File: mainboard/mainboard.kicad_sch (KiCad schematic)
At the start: 46 parts, among them J1 Conn_01x14, J2 Conn_02x06_Top_Bottom, J3 OLED, J6 Conn_01x05, J7 SHF-105-01-L-D-RA, SW35 SW_Push, SW36 SW_Push, U1 RP2350A, U2 W25Q128JVSIQ, Y1 ABM8-272-T3

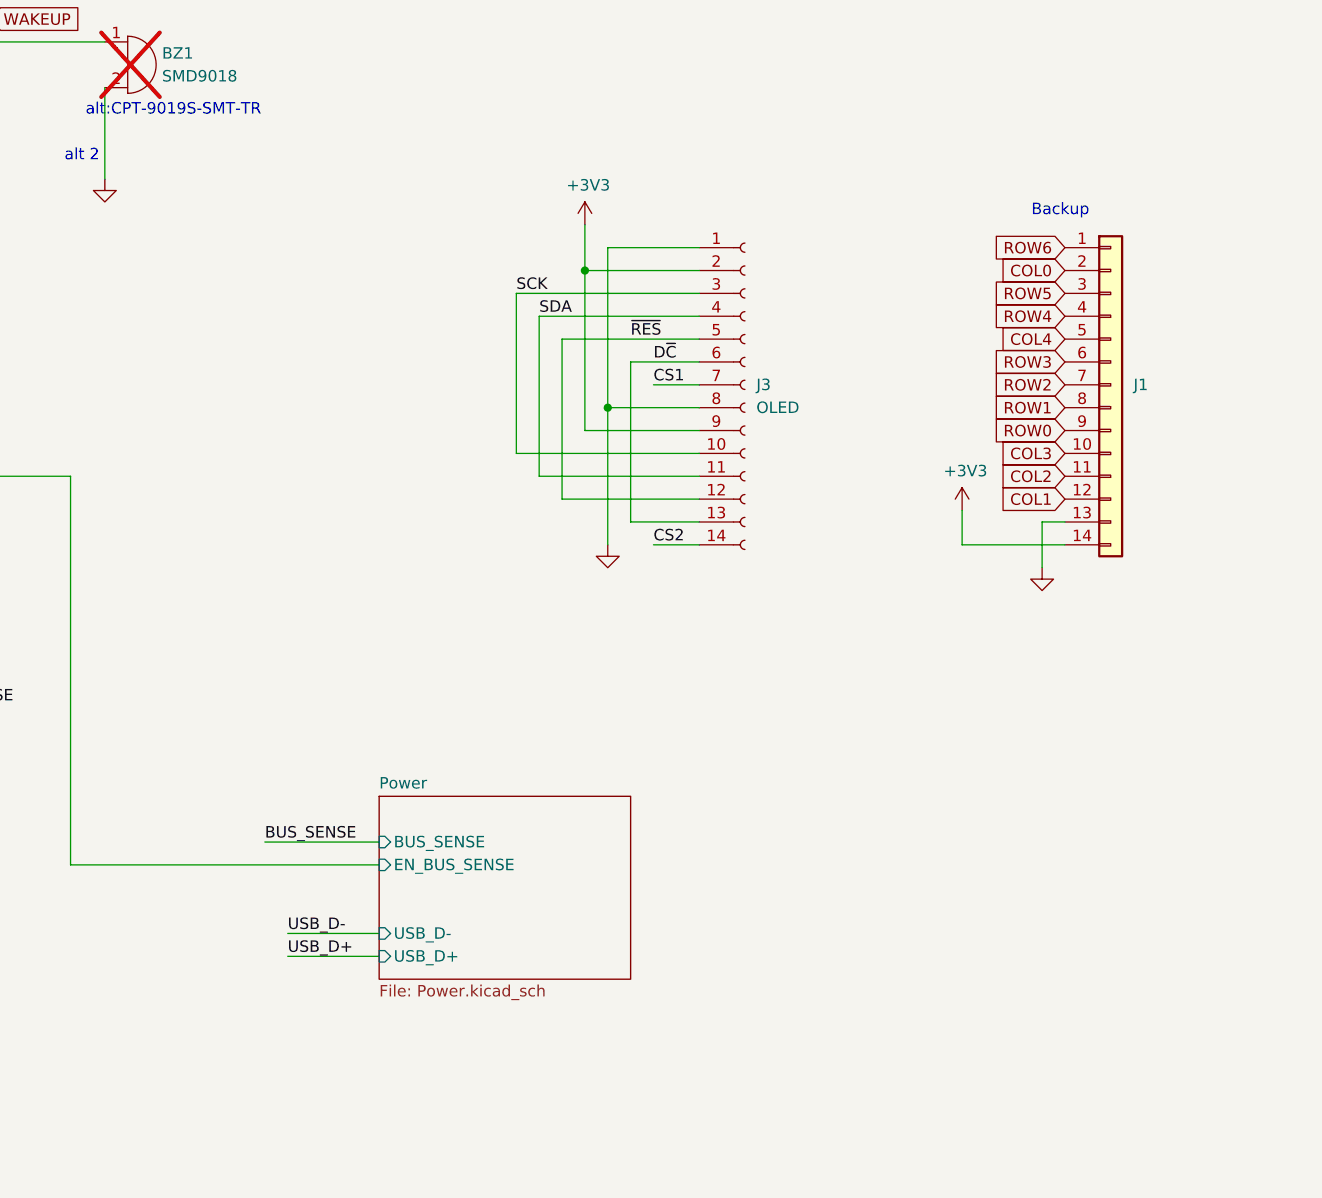
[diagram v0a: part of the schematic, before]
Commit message: keyboard done
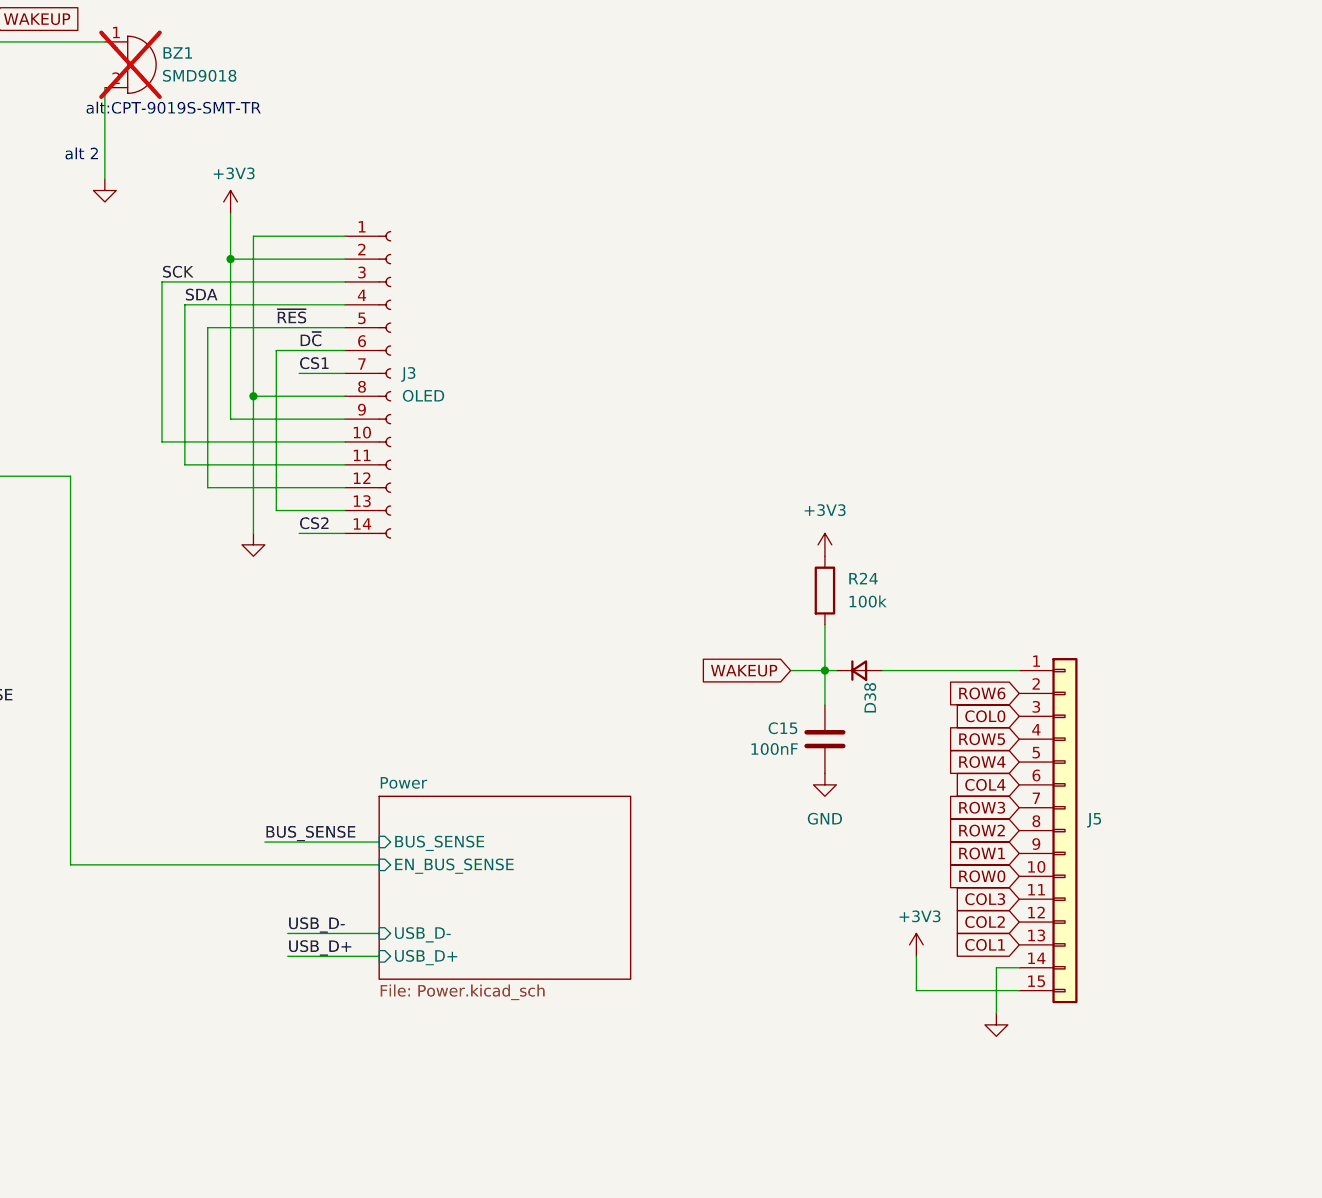
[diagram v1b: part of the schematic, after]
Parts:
- removed J1: Conn_01x14, Connector_PinHeader_2.54mm:PinHeader_1x14_P2.54mm_Vertical, symbol Connector_Generic:Conn_01x14
- added C15: 100nF, Capacitor_SMD:C_0402_1005Metric, symbol Device:C
- added D38: D, Diode_SMD:D_SOD-323, symbol Device:D_Small
- added J5: Conn_01x15, Connector_PinHeader_2.54mm:PinHeader_1x15_P2.54mm_Vertical, symbol Connector_Generic:Conn_01x15
- added R24: 100k, Resistor_SMD:R_0402_1005Metric, symbol Device:R
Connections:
- net +3V3: now also J5.15 (Pin_15), R24.1
- net COL0: now also J5.3 (Pin_3)
- net COL1: now also J5.13 (Pin_13)
- net COL2: now also J5.12 (Pin_12)
- net COL3: now also J5.11 (Pin_11)
- net COL4: now also J5.6 (Pin_6)
- net GND: now also C15.2, J5.14 (Pin_14)
- net ROW0: now also J5.10 (Pin_10)
- net ROW1: now also J5.9 (Pin_9)
- net ROW2: now also J5.8 (Pin_8)
- net ROW3: now also J5.7 (Pin_7)
- net ROW4: now also J5.5 (Pin_5)
- net ROW5: now also J5.4 (Pin_4)
- net ROW6: now also J5.2 (Pin_2)
- net WAKEUP: now also C15.1, D38.1 (K), R24.2
- new net: D38.2 (A), J5.1 (Pin_1)
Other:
- note removed: "Backup"
- moved on the sheet: J3
